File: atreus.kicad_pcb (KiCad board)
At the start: 2 copper layers, 139.7 x 101.6 mm, 45 parts

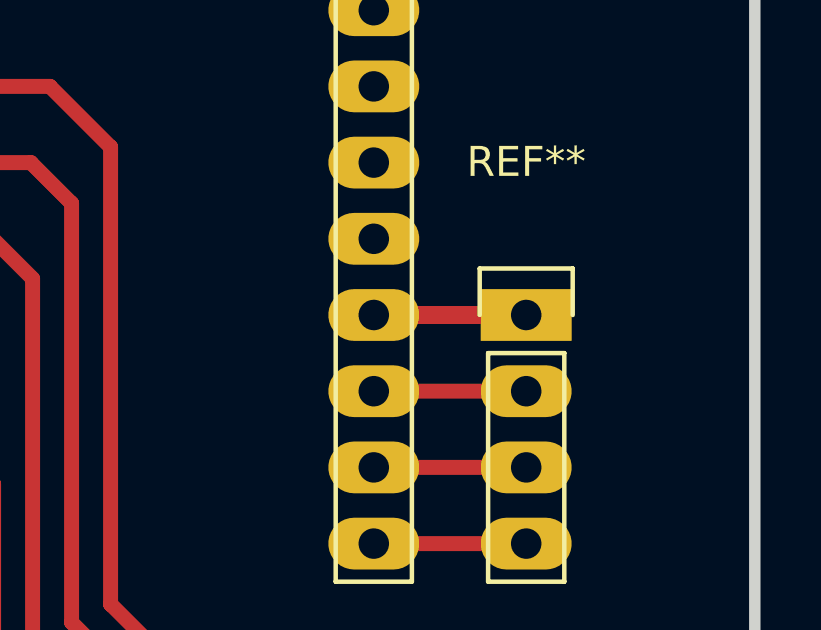
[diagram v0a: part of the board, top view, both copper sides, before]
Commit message: c
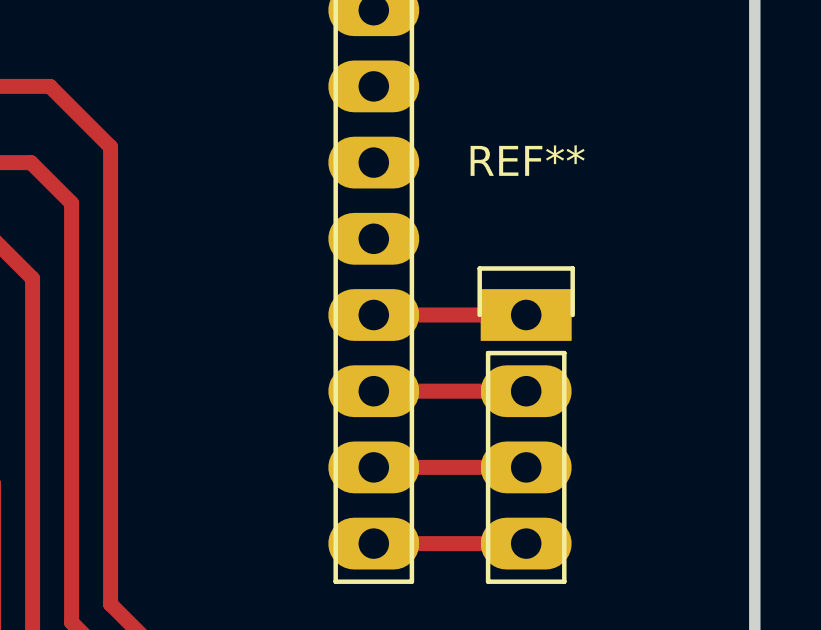
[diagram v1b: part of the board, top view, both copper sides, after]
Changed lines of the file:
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@@
     (mod_text_size 1.524 1.524)
     (mod_text_width 0.3048)
-    (pad_size 2.5 1.651)
-    (pad_drill 0.9906)
+    (pad_size 3.032 1.7272)
+    (pad_drill 1.016)
     (pad_to_mask_clearance 0.254)
     (aux_axis_origin 0 0)
@@
   (segment (start 144.78 63.5) (end 149.86 63.5) (width 0.5) (layer Front) (net 0))
   (segment (start 144.78 60.96) (end 149.86 60.96) (width 0.5) (layer Front) (net 0))
-  (segment (start 144.78 58.42) (end 149.86 58.42) (width 0.6) (layer Front) (net 0))
+  (segment (start 144.78 58.42) (end 149.86 58.42) (width 0.5) (layer Front) (net 0))
   (segment (start 124 37.005) (end 125.095 38.1) (width 0.5) (layer Front) (net 1))
   (segment (start 125.095 38.1) (end 129.54 38.1) (width 0.5) (layer Front) (net 1))
